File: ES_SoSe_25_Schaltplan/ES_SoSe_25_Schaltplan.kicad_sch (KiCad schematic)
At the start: 8 parts

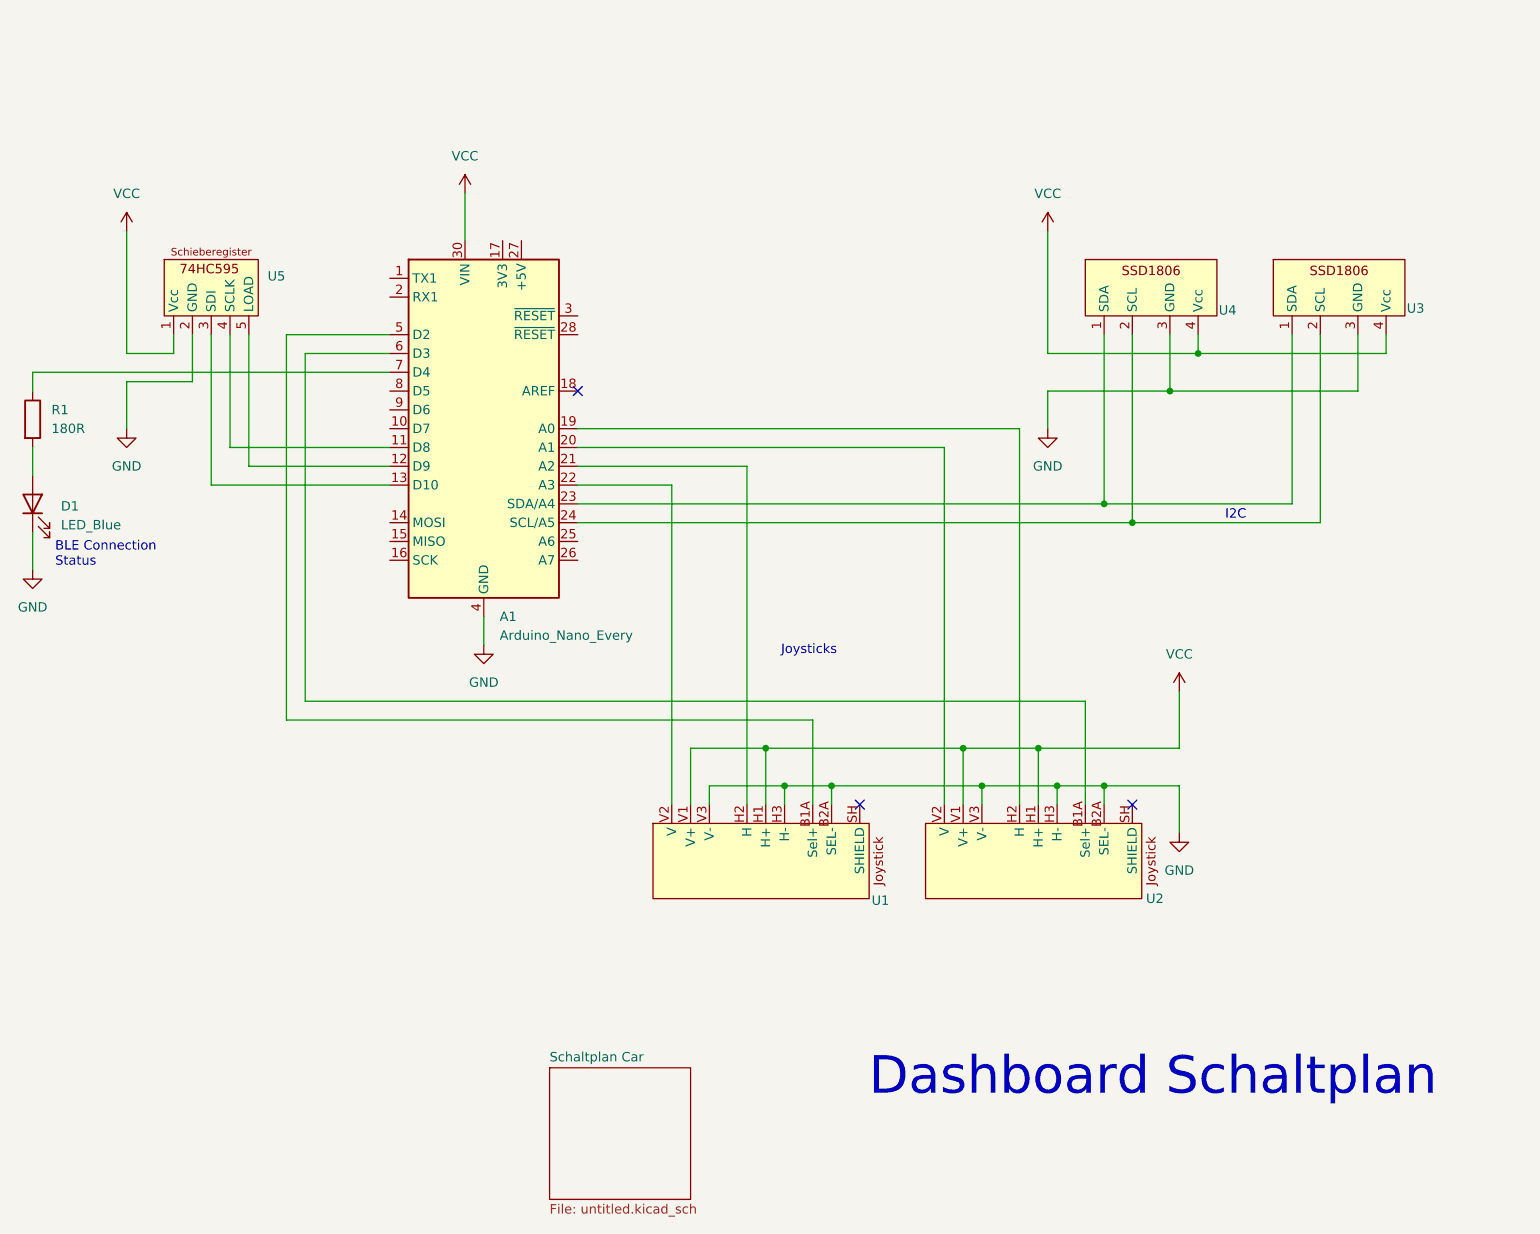
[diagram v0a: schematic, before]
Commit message: updated scematic
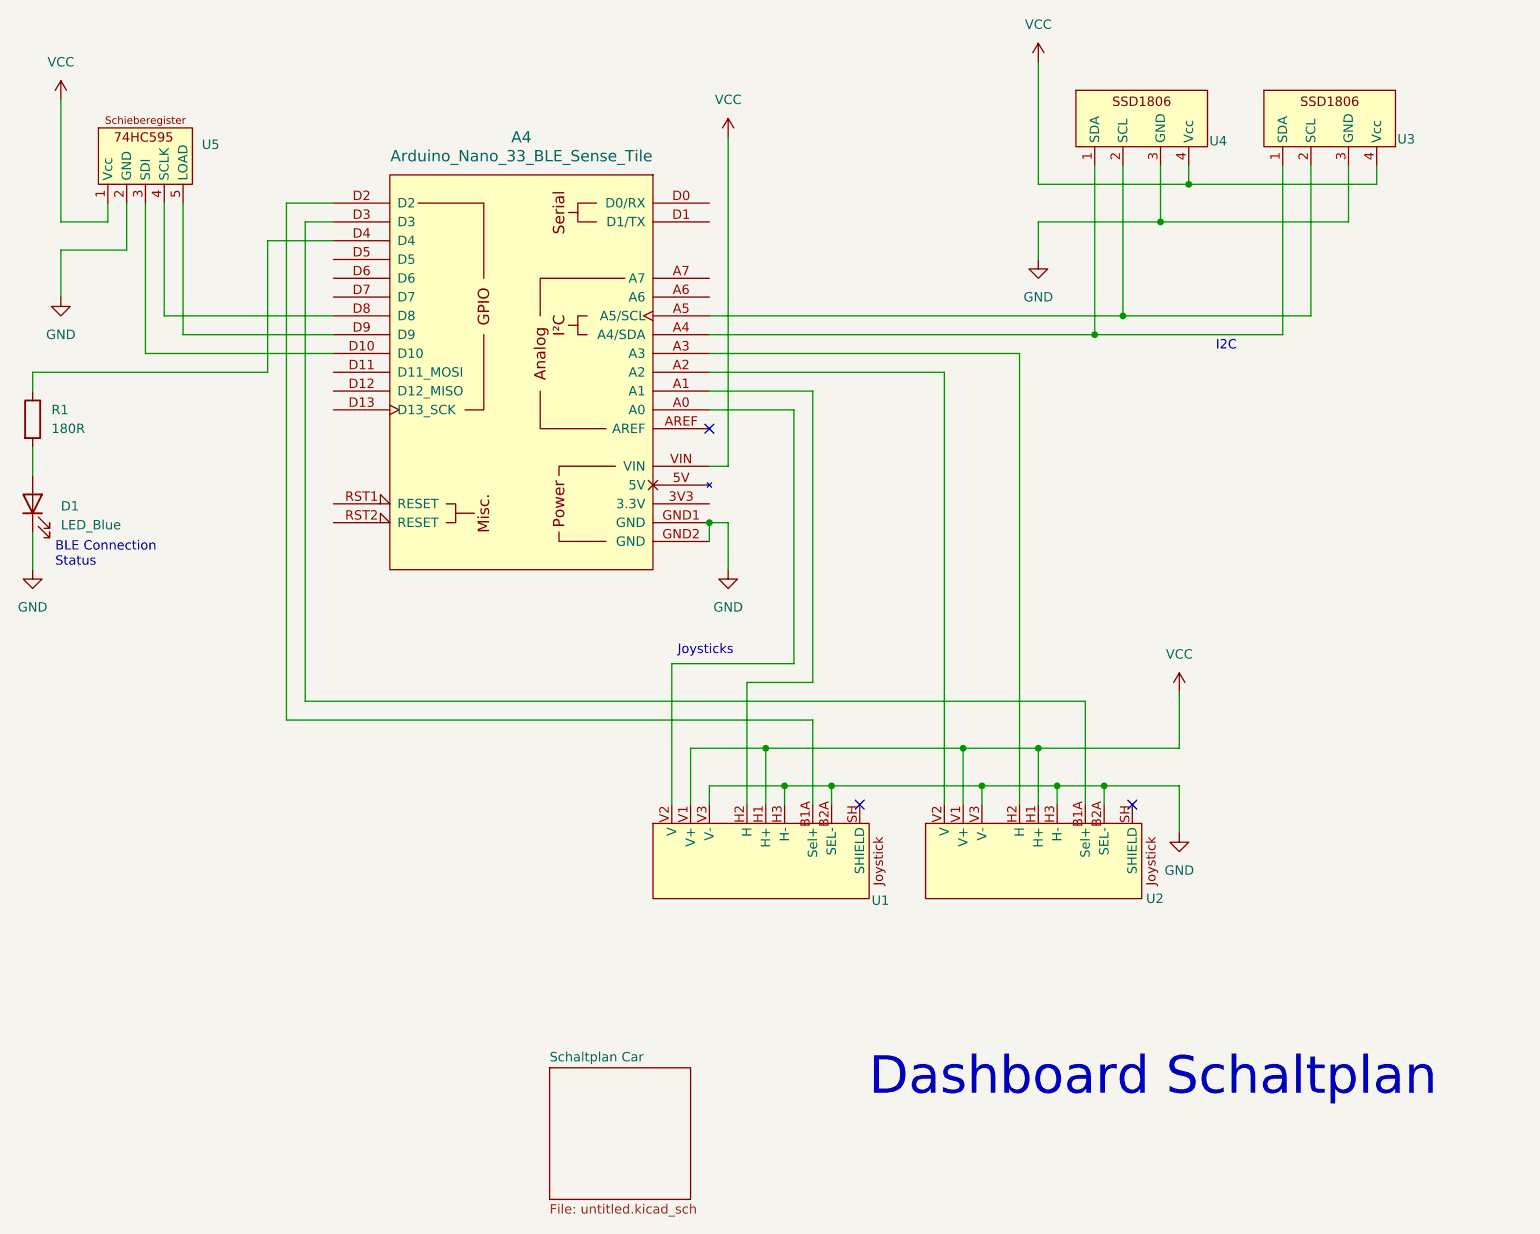
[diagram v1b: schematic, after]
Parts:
- removed A1: Arduino_Nano_Every, Module:Arduino_Nano, symbol MCU_Module:Arduino_Nano_Every
- added A4: Arduino_Nano_33_BLE_Sense_Tile, PCM_arduino-library:Arduino_Nano_Every_Tile, symbol arduino-library:Arduino_Nano_33_BLE_Sense_Tile
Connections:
- net GND: now also A4.GND1 (GND), A4.GND2 (GND)
- net VCC: now also A4.VIN
- net at R1.1: now also A4.D4
- net at U5.4 (SCLK): now also A4.D8
- net at U5.5 (LOAD): now also A4.D9
- net at U5.3 (SDI): now also A4.D10
- net at U2.H2 (H): now also A4.A3
- net at U2.V2 (V): now also A4.A2
- net at U1.H2 (H): now also A4.A1
- net at U1.V2 (V): now also A4.A0
- net at U3.1 (SDA), U4.1 (SDA): now also A4.A4 (A4/SDA)
- net at U3.2 (SCL), U4.2 (SCL): now also A4.A5 (A5/SCL)
- net at U1.B1A (Sel+): now also A4.D2
- net at U2.B1A (Sel+): now also A4.D3
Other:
- moved on the sheet: U3, U4, U5
